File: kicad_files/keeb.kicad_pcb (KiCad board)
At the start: 2 copper layers, 369.3 x 148.8 mm, 232 parts, among them SW10 SW_Push, SW11 SW_Push, SW12 SW_Push, SW13 SW_Push, SW14 SW_Push, SW15 SW_Push, SW16 SW_Push, SW17 SW_Push, SW18 SW_Push, SW19 SW_Push, SW2 RotaryEncoder_Switch, SW20 SW_Push, SW21 SW_Push, SW22 SW_Push, SW23 SW_Push, SW24 SW_Push, SW25 SW_Push, SW26 SW_Push, SW27 SW_Push, SW28 SW_Push, SW29 SW_Push, SW3 SW_Push, SW30 SW_Push, SW31 SW_Push, SW32 SW_Push, SW33 SW_Push, SW34 SW_Push, SW35 SW_Push, SW36 SW_Push, SW37 SW_Push, SW38 SW_Push, SW39 SW_Push, SW4 SW_Push, SW40 SW_Push, SW41 SW_Push, SW42 SW_Push, SW43 SW_Push, SW44 SW_Push, SW45 SW_Push, SW46 SW_Push, SW47 SW_Push, SW48 SW_Push, SW49 SW_Push, SW5 SW_Push, SW50 SW_Push, SW51 SW_Push, SW52 SW_Push, SW53 SW_Push, SW54 SW_Push, SW55 SW_Push, SW56 SW_Push, SW6 SW_Push, SW7 SW_Push, SW8 SW_Push, SW9 SW_Push, U2 ER_OLEDM0.91_1x-I2C

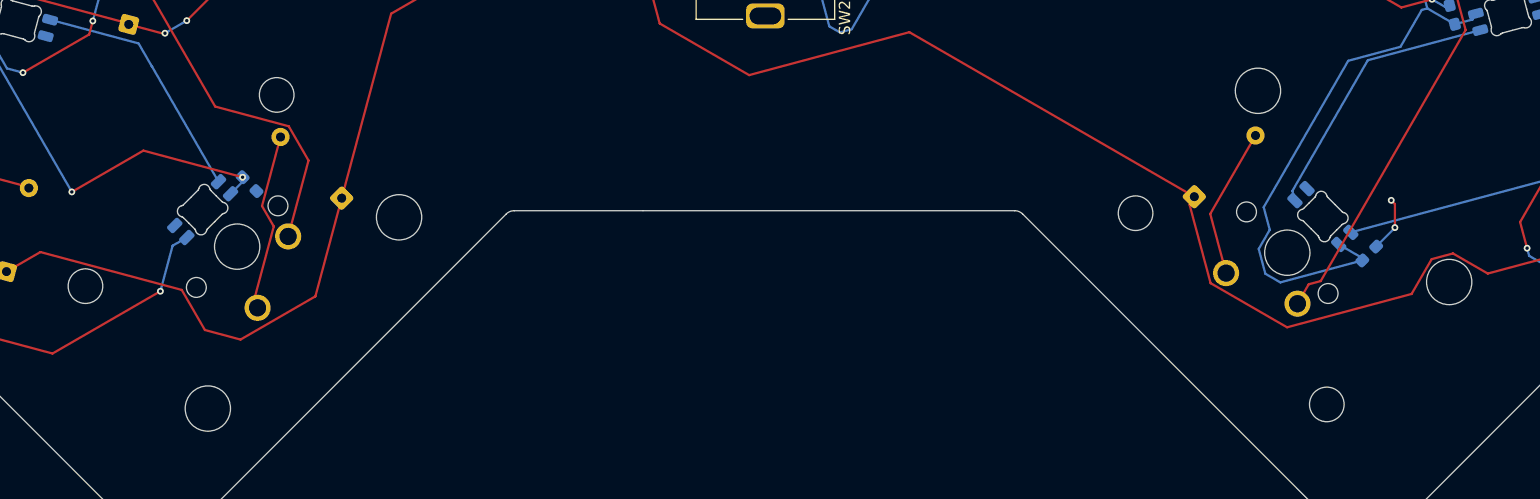
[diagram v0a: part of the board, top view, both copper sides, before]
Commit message: Journal Fix
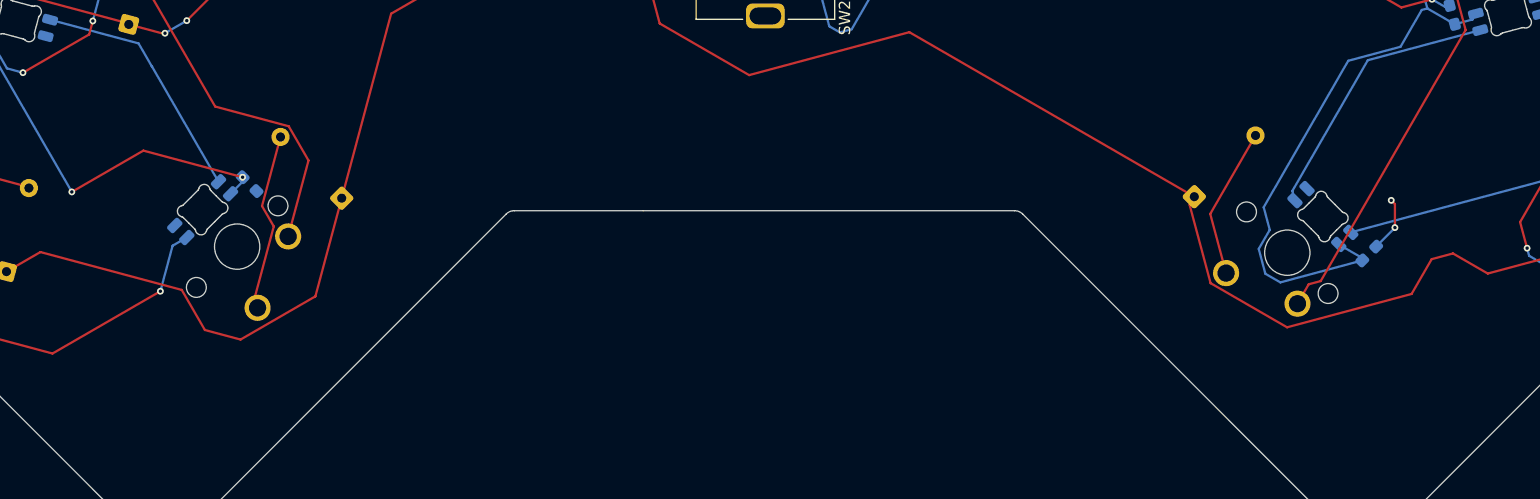
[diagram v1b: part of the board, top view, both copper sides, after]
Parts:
- removed S1, S2: MX_stab, PCM_marbastlib-mx:STAB_MX_2u
